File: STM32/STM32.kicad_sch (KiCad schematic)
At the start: 1 part, among them U1 STM32F103C8Tx

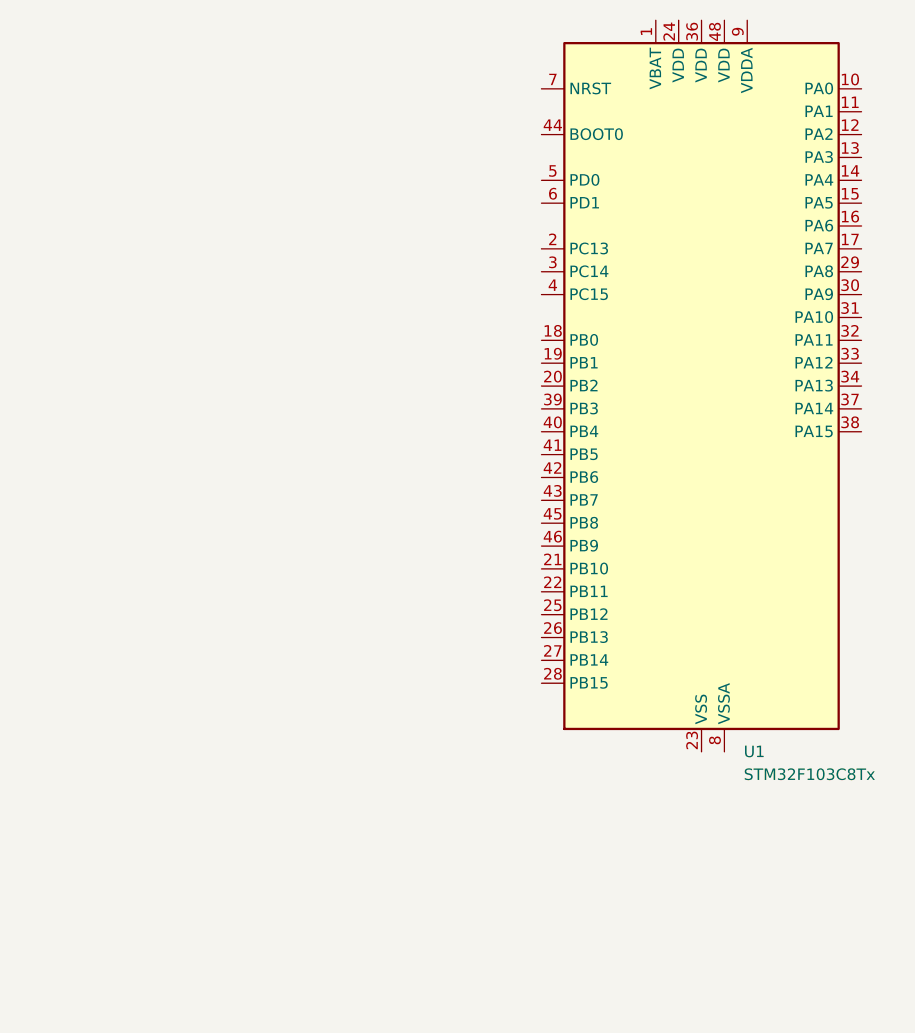
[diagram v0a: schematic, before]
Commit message: completed pcb routing
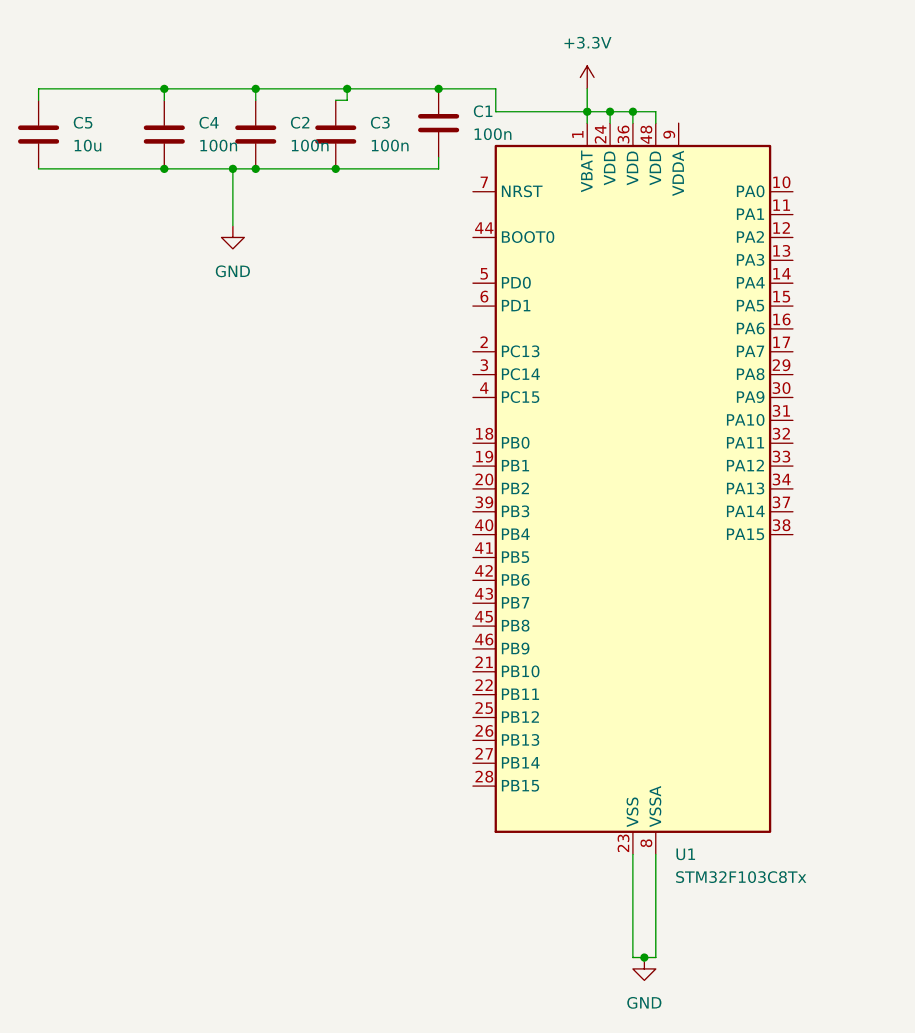
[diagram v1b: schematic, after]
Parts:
- added C1, C2, C3, C4: 100n, symbol Device:C
- added C5: 10u, symbol Device:C
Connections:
- net +3.3V: now reaches U1.1 (VBAT)
- net +3.3V: now also U1.24 (VDD), U1.36 (VDD), U1.48 (VDD), C1.1, C2.1, C3.1, C4.1, C5.1
- net GND: now reaches U1.23 (VSS), U1.35 (VSS), U1.47 (VSS)
- net GND: now also U1.8 (VSSA), C1.2, C2.2, C3.2, C4.2, C5.2
